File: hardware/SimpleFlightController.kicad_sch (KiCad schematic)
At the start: 39 parts, among them J1 Screw_Terminal_01x02, U1 BQ25883RGER, U2 ICM-45686, U3 STM32F722RETx, U4 BMP580, U5 TPS63070RNMR, U6 LMR51430

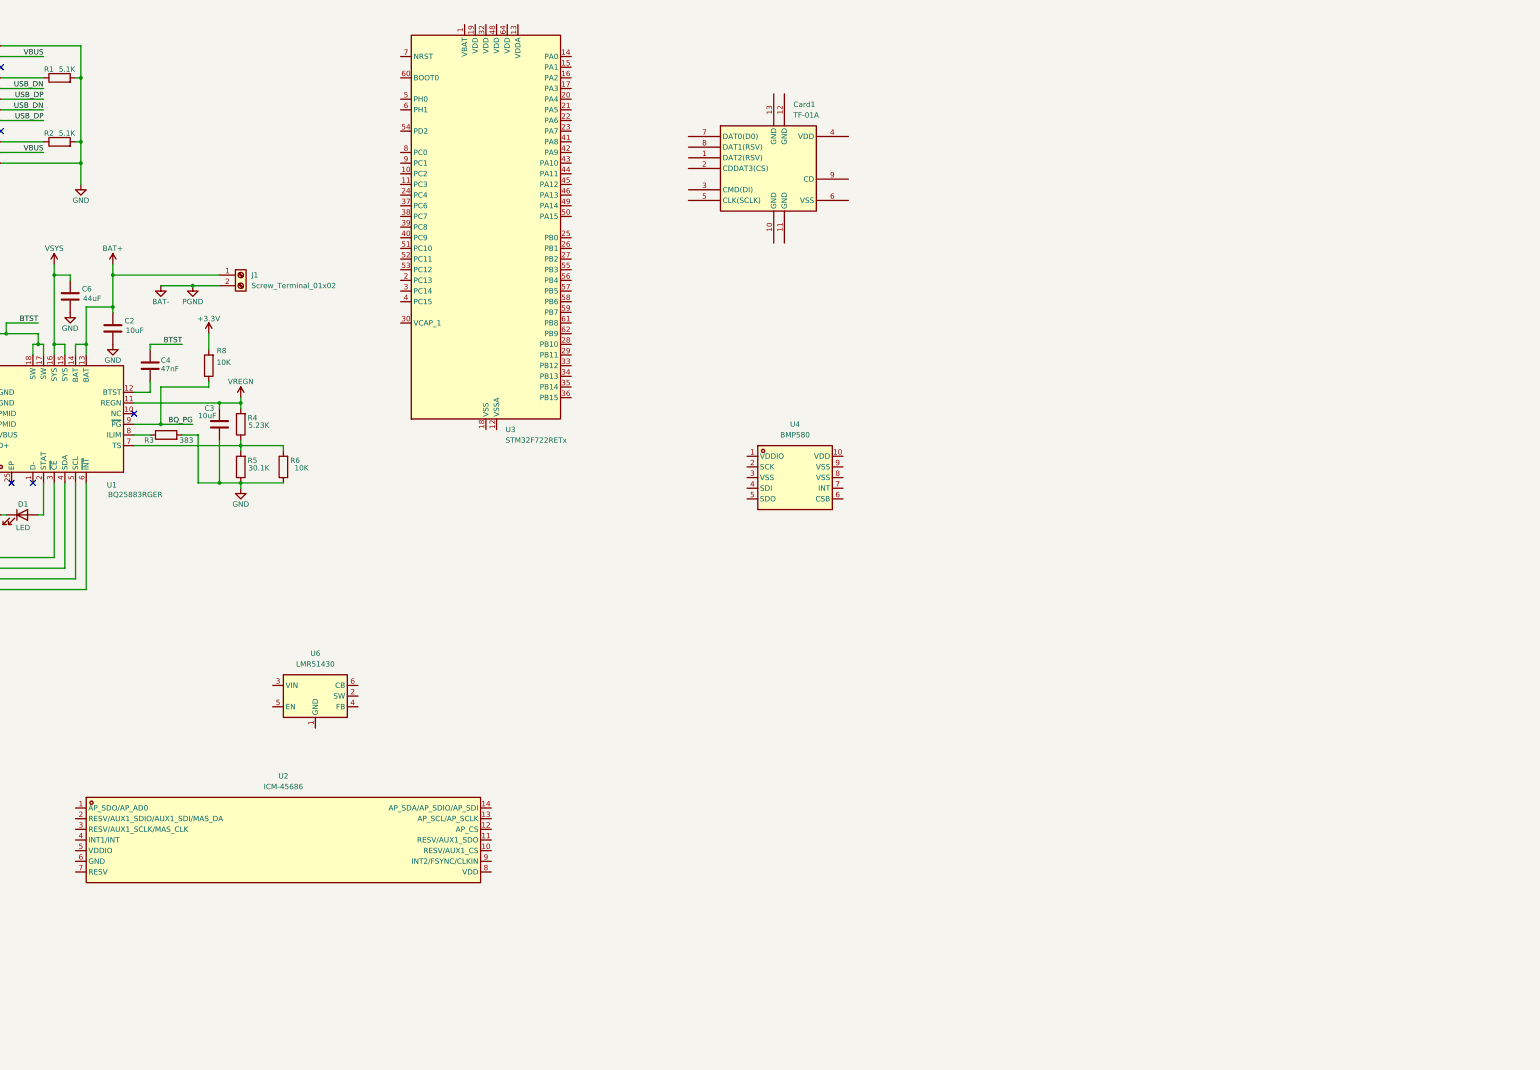
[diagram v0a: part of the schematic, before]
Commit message: added more stuff
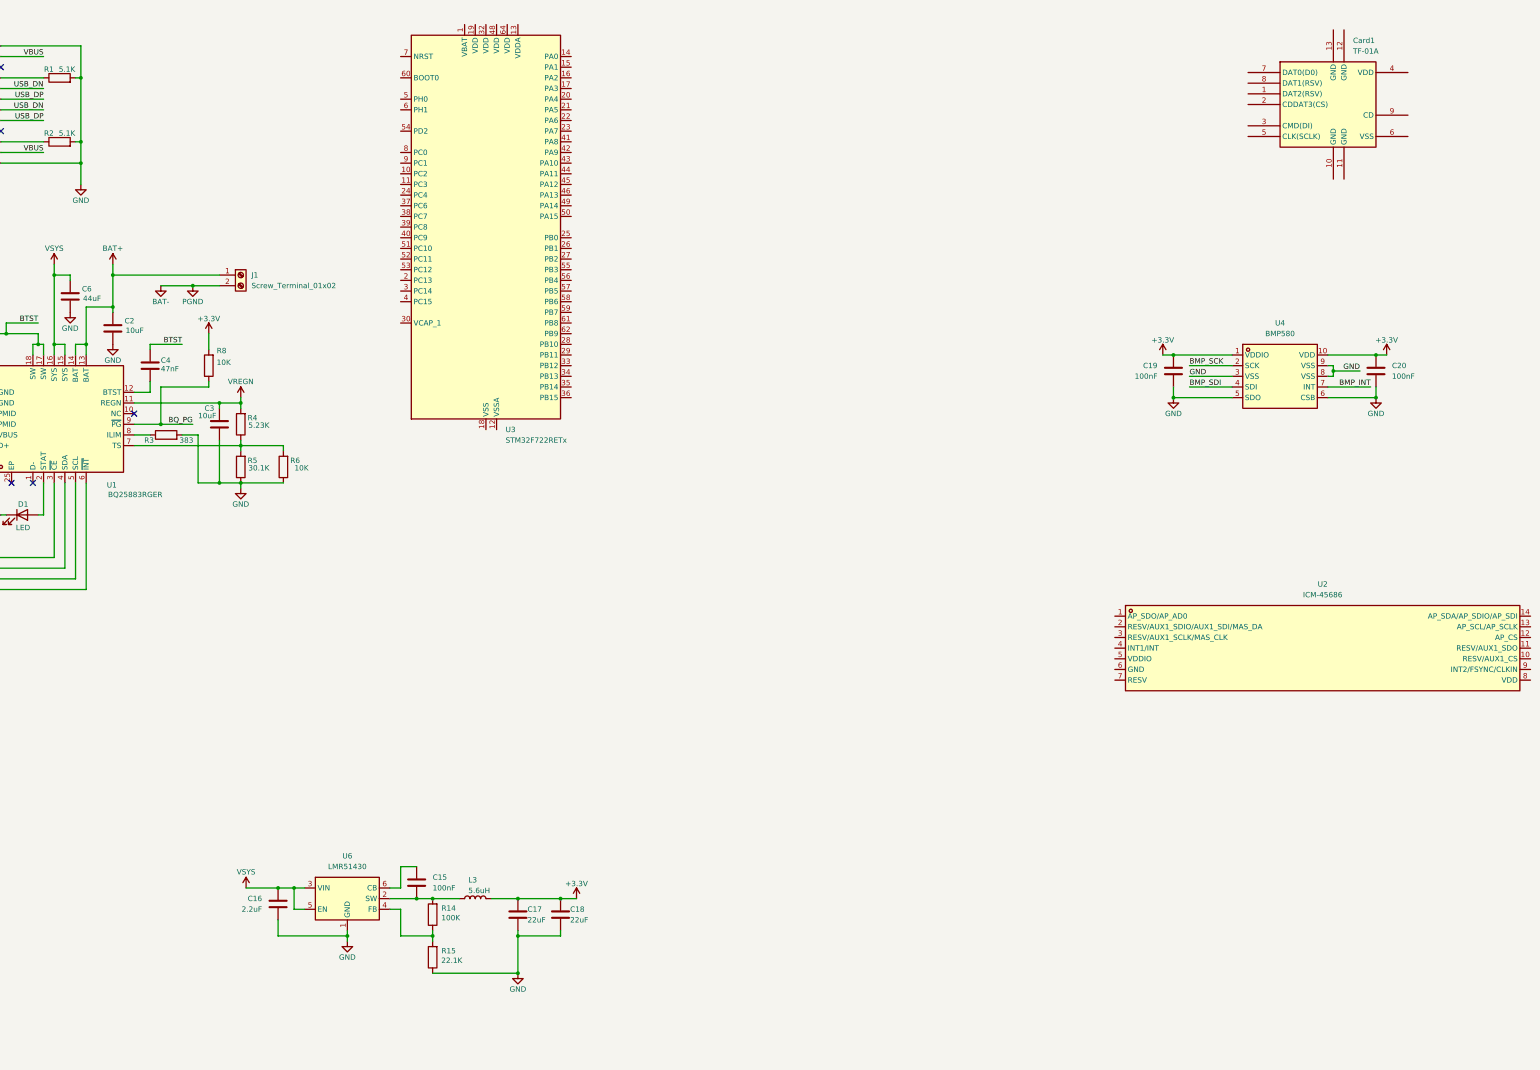
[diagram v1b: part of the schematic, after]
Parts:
- added C15, C19, C20: 100nF, symbol Device:C
- added C16: 2.2uF, symbol Device:C
- added C17, C18: 22uF, symbol Device:C
- added L3: 5.6uH, symbol Device:L
- added R14: 100K, symbol Device:R
- added R15: 22.1K, symbol Device:R
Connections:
- net +3.3V: now also U4.1 (VDDIO), U4.10 (VDD), C17.1, C18.1, C19.1, C20.1, L3.2
- net GND: now also U4.3 (VSS), U4.5 (SDO), U4.6 (CSB), U4.8 (VSS), U4.9 (VSS), U6.1 (GND), C16.2, C17.2, C18.2, C19.2, C20.2, R15.1
- net VSYS: now also U6.3 (VIN), U6.5 (EN), C16.1
- net at U6.2 (SW): now also C15.2, L3.1, R14.2
- net at U6.4 (FB): now also R14.1, R15.2
- net at U6.6 (CB): now also C15.1
- net BMP_SCK: now reaches U4.2 (SCK)
- net BMP_SDI: now reaches U4.4 (SDI)
- net BMP_INT: now reaches U4.7 (INT)
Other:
- moved on the sheet: Card1, U2, U4, U6
